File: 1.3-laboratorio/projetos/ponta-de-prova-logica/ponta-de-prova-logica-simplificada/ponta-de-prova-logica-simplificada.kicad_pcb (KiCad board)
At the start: 2 copper layers, 64.8 x 40 mm, 21 parts, among them J1 Conn_01x02, J2 PONTA DE PROVA, SW1 SW_DPDT_x2, U1 LM339

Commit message: Arquivos PDF para confecção da placa.
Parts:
- D1: value LED ALTO -> ALTO
- D2: value LED BAIXO -> BAIXO
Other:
- board text added: "2x 820/0.5W"

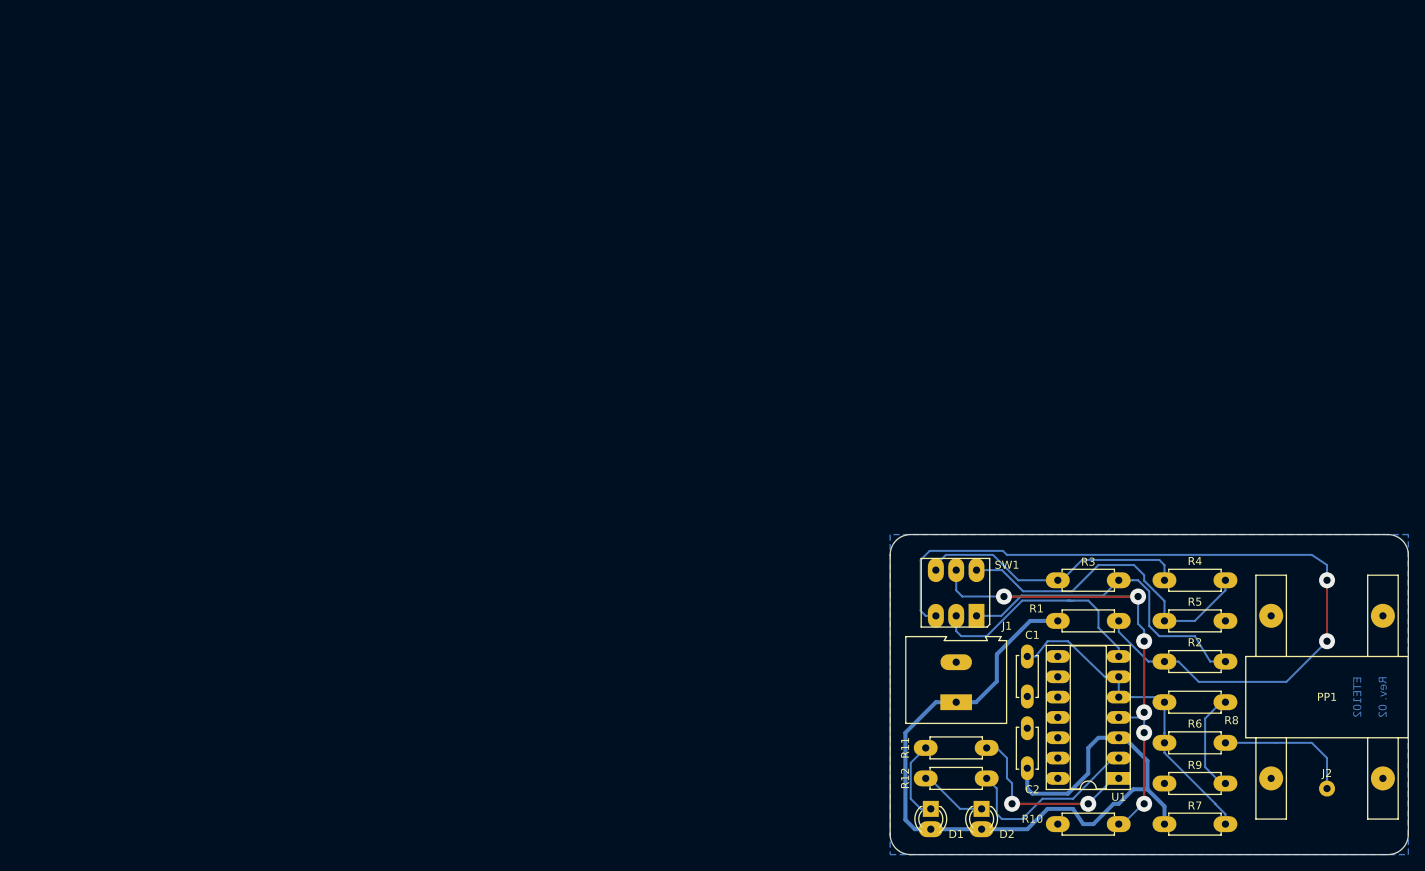
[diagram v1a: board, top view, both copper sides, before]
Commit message: Arquivos para impressão de fotolito preparados.
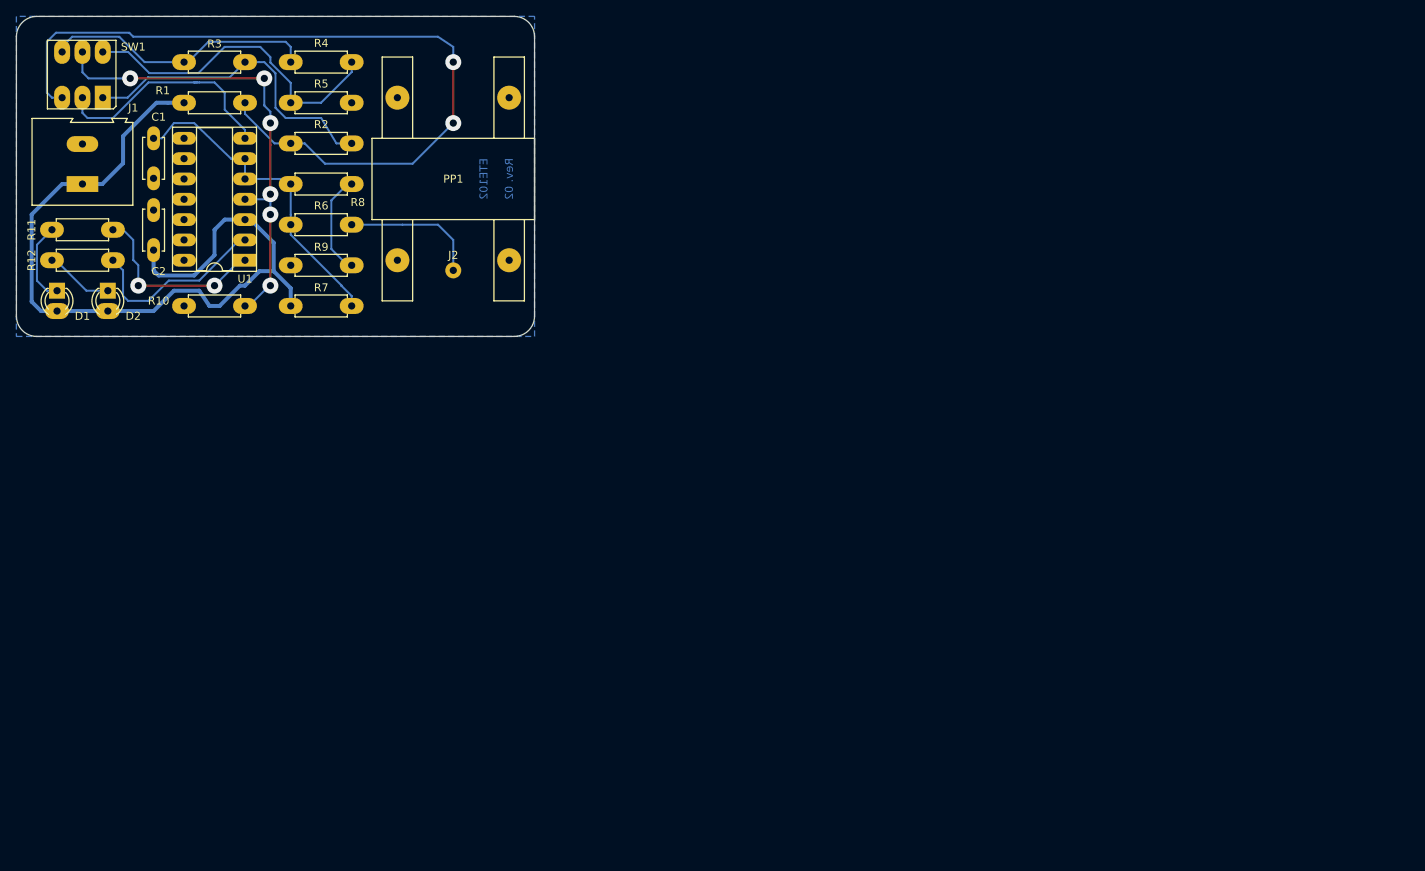
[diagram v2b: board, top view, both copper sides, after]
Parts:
- moved C1 127.0 mm to (31.1, 29.8)
- moved C2 127.0 mm to (31.1, 43.8)
- moved D1 127.0 mm to (19.1, 48.9)
- moved J2 127.0 mm to (68.6, 46.4)
- moved R1 127.0 mm to (34.9, 25.4)
- moved D2 127.0 mm to (25.4, 48.9)
- moved J1 127.0 mm to (22.2, 35.6)
- moved R11 127.0 mm to (18.4, 41.3)
- moved R12 127.0 mm to (18.4, 45.1)
- moved R2 127.0 mm to (48.3, 30.5)
- moved R4 127.0 mm to (48.3, 20.3)
- moved R5 127.0 mm to (48.3, 25.4)
- moved R6 127.0 mm to (48.3, 40.6)
- moved R7 127.0 mm to (48.3, 50.8)
- moved R8 127.0 mm to (48.3, 35.6)
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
